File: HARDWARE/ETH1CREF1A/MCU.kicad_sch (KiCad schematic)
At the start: 42 parts, among them J1001 Conn_02x01, J1002 20021111-00010T4LF, U1001 HDC1080, U1002 STM32F746ZG, U1003 24LC08B-E/MS, Y1001 NX5032GA-16.000M

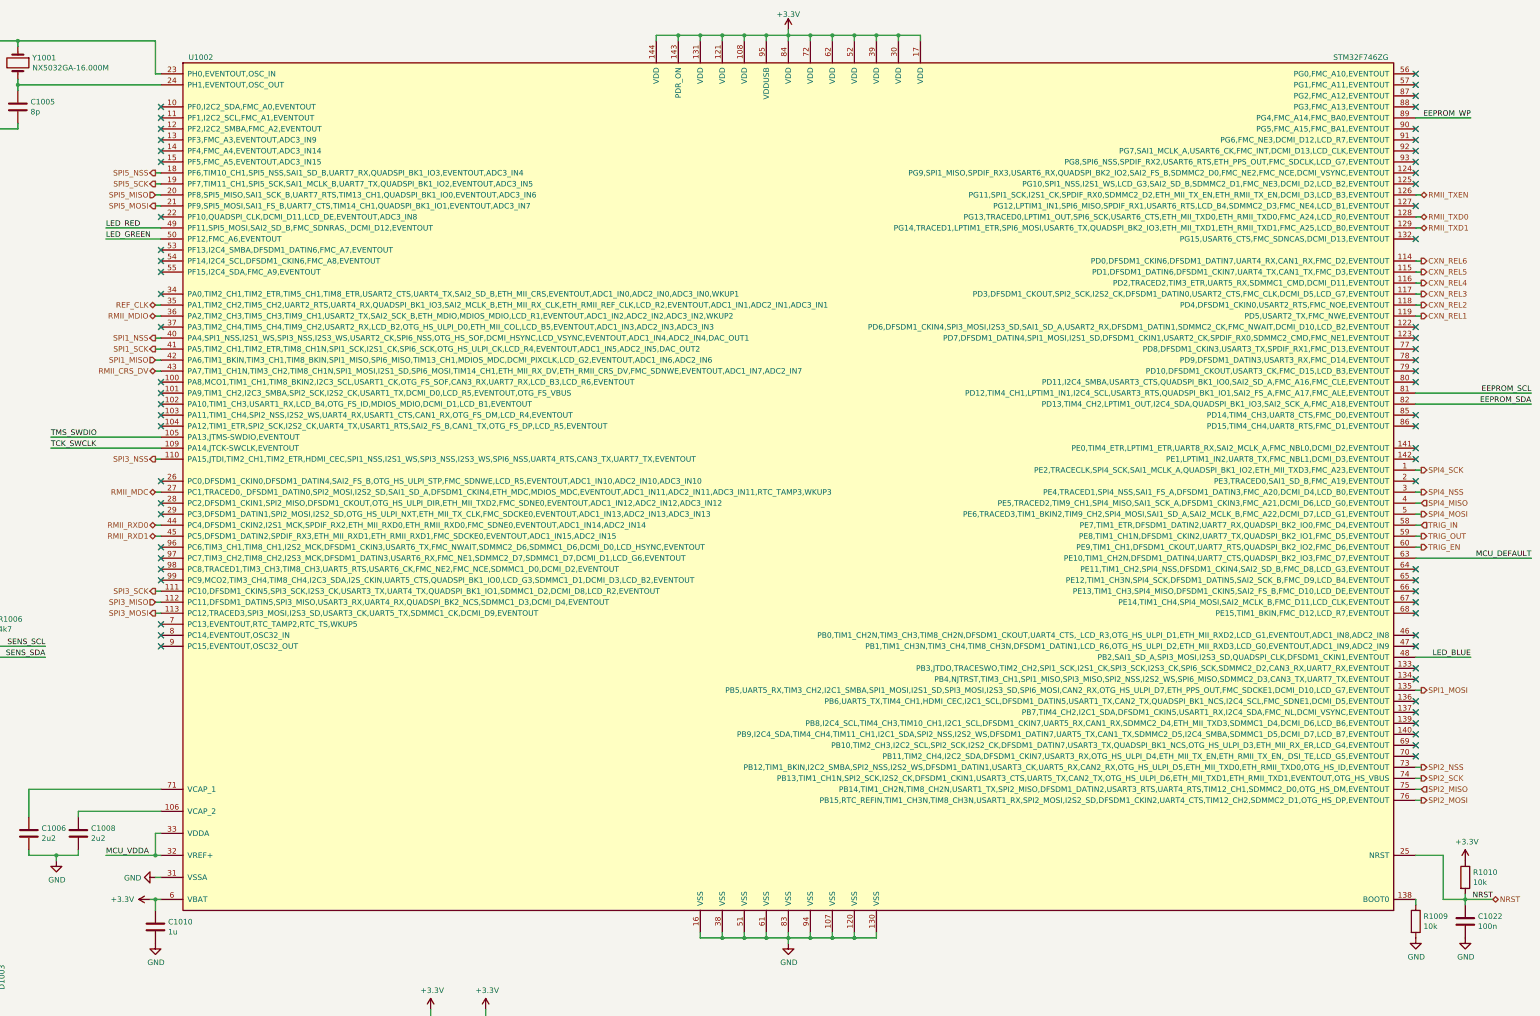
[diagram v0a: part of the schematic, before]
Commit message: Hardware and software
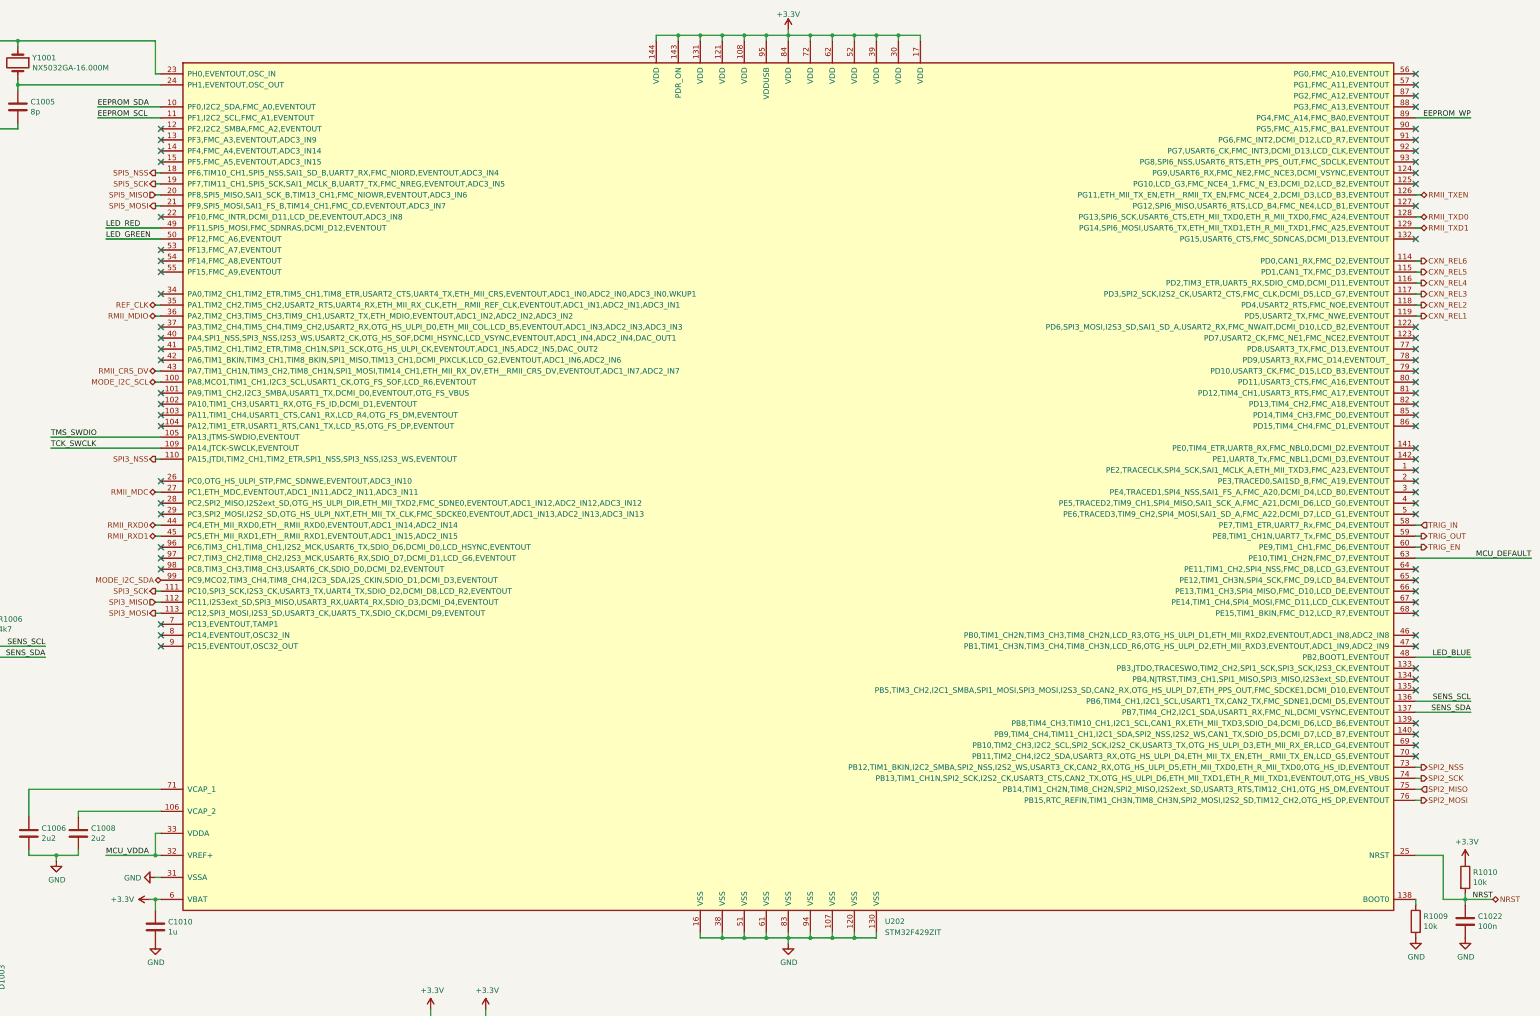
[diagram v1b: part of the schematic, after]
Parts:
- removed U1002: STM32F746ZG, ETH1CREF1A:TQFP-144_20x20mm_P0.5mm, symbol ETH1CSMU2:STM32F746ZG
- added U202: STM32F429ZIT, ETH1CREF1A:TQFP-144_20x20mm_P0.5mm, symbol ETH1CREF1A:STM32F429ZIT
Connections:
- net +3.3V: now also U202.108 (VDD), U202.121 (VDD), U202.131 (VDD), U202.143 (PDR_ON), U202.144 (VDD), U202.17 (VDD), U202.30 (VDD), U202.39 (VDD), U202.52 (VDD), U202.6 (VBAT), U202.62 (VDD), U202.72 (VDD), U202.84 (VDD), U202.95 (VDDUSB)
- net CXN_REL1: now also U202.119 (PD5,USART2_TX,FMC_NWE,EVENTOUT)
- net CXN_REL2: now also U202.118 (PD4,USART2_RTS,FMC_NOE,EVENTOUT)
- net CXN_REL3: now also U202.117 (PD3,SPI2_SCK,I2S2_CK,USART2_CTS,FMC_CLK,DCMI_D5,LCD_G7,EVENTOUT)
- net CXN_REL4: now also U202.116 (PD2,TIM3_ETR,UART5_RX,SDIO_CMD,DCMI_D11,EVENTOUT)
- net CXN_REL5: now also U202.115 (PD1,CAN1_TX,FMC_D3,EVENTOUT)
- net CXN_REL6: now also U202.114 (PD0,CAN1_RX,FMC_D2,EVENTOUT)
- net EEPROM_SCL: now also U202.11 (PF1,I2C2_SCL,FMC_A1,EVENTOUT)
- net EEPROM_SDA: now also U202.10 (PF0,I2C2_SDA,FMC_A0,EVENTOUT)
- net EEPROM_WP: now also U202.89 (PG4,FMC_A14,FMC_BA0,EVENTOUT)
- net GND: now also U202.107 (VSS), U202.120 (VSS), U202.130 (VSS), U202.16 (VSS), U202.31 (VSSA), U202.38 (VSS), U202.51 (VSS), U202.61 (VSS), U202.83 (VSS), U202.94 (VSS)
- net LED_BLUE: now also U202.48 (PB2,BOOT1,EVENTOUT)
- net LED_GREEN: now also U202.50 (PF12,FMC_A6,EVENTOUT)
- net LED_RED: now also U202.49 (PF11,SPI5_MOSI,FMC_SDNRAS,DCMI_D12,EVENTOUT)
- net MCU_DEFAULT: now also U202.63 (PE10,TIM1_CH2N,FMC_D7,EVENTOUT)
- net MCU_VDDA: now also U202.32 (VREF+), U202.33 (VDDA)
- net NRST: now also U202.25 (NRST)
- net REF_CLK: now also U202.35 (PA1,TIM2_CH2,TIM5_CH2,USART2_RTS,UART4_RX,ETH_MII_RX_CLK,ETH__RMII_REF_CLK,EVENTOUT,ADC1_IN1,ADC2_IN1,ADC3_IN1)
- net RMII_CRS_DV: now also U202.43 (PA7,TIM1_CH1N,TIM3_CH2,TIM8_CH1N,SPI1_MOSI,TIM14_CH1,ETH_MII_RX_DV,ETH__RMII_CRS_DV,EVENTOUT,ADC1_IN7,ADC2_IN7)
- net RMII_MDC: now also U202.27 (PC1,ETH_MDC,EVENTOUT,ADC1_IN11,ADC2_IN11,ADC3_IN11)
- net RMII_MDIO: now also U202.36 (PA2,TIM2_CH3,TIM5_CH3,TIM9_CH1,USART2_TX,ETH_MDIO,EVENTOUT,ADC1_IN2,ADC2_IN2,ADC3_IN2)
- net RMII_RXD0: now also U202.44 (PC4,ETH_MII_RXD0,ETH__RMII_RXD0,EVENTOUT,ADC1_IN14,ADC2_IN14)
- net RMII_RXD1: now also U202.45 (PC5,ETH_MII_RXD1,ETH__RMII_RXD1,EVENTOUT,ADC1_IN15,ADC2_IN15)
- net RMII_TXD0: now also U202.128 (PG13,SPI6_SCK,USART6_CTS,ETH_MII_TXD0,ETH_R_MII_TXD0,FMC_A24,EVENTOUT)
- net RMII_TXD1: now also U202.129 (PG14,SPI6_MOSI,USART6_TX,ETH_MII_TXD1,ETH_R_MII_TXD1,FMC_A25,EVENTOUT)
- net RMII_TXEN: now also U202.126 (PG11,ETH_MII_TX_EN,ETH__RMII_TX_EN,FMC_NCE4_2,DCMI_D3,LCD_B3,EVENTOUT)
- net SENS_SCL: now also U202.136 (PB6,TIM4_CH1,I2C1_SCL,USART1_TX,CAN2_TX,FMC_SDNE1,DCMI_D5,EVENTOUT)
- net SENS_SDA: now also U202.137 (PB7,TIM4_CH2,I2C1_SDA,USART1_RX,FMC_NL,DCMI_VSYNC,EVENTOUT)
- net SPI2_MISO: now also U202.75 (PB14,TIM1_CH2N,TIM8_CH2N,SPI2_MISO,I2S2ext_SD,USART3_RTS,TIM12_CH1,OTG_HS_DM,EVENTOUT)
- net SPI2_MOSI: now also U202.76 (PB15,RTC_REFIN,TIM1_CH3N,TIM8_CH3N,SPI2_MOSI,I2S2_SD,TIM12_CH2,OTG_HS_DP,EVENTOUT)
- net SPI2_NSS: now also U202.73 (PB12,TIM1_BKIN,I2C2_SMBA,SPI2_NSS,I2S2_WS,USART3_CK,CAN2_RX,OTG_HS_ULPI_D5,ETH_MII_TXD0,ETH_R_MII_TXD0,OTG_HS_ID,EVENTOUT)
- net SPI2_SCK: now also U202.74 (PB13,TIM1_CH1N,SPI2_SCK,I2S2_CK,USART3_CTS,CAN2_TX,OTG_HS_ULPI_D6,ETH_MII_TXD1,ETH_R_MII_TXD1,EVENTOUT,OTG_HS_VBUS)
- net SPI3_MISO: now also U202.112 (PC11,I2S3ext_SD,SPI3_MISO,USART3_RX,UART4_RX,SDIO_D3,DCMI_D4,EVENTOUT)
- net SPI3_MOSI: now also U202.113 (PC12,SPI3_MOSI,I2S3_SD,USART3_CK,UART5_TX,SDIO_CK,DCMI_D9,EVENTOUT)
- net SPI3_NSS: now also U202.110 (PA15,JTDI,TIM2_CH1,TIM2_ETR,SPI1_NSS,SPI3_NSS,I2S3_WS,EVENTOUT)
- net SPI3_SCK: now also U202.111 (PC10,SPI3_SCK,I2S3_CK,USART3_TX,UART4_TX,SDIO_D2,DCMI_D8,LCD_R2,EVENTOUT)
- net SPI5_MISO: now also U202.20 (PF8,SPI5_MISO,SAI1_SCK_B,TIM13_CH1,FMC_NIOWR,EVENTOUT,ADC3_IN6)
- net SPI5_MOSI: now also U202.21 (PF9,SPI5_MOSI,SAI1_FS_B,TIM14_CH1,FMC_CD,EVENTOUT,ADC3_IN7)
- net SPI5_NSS: now also U202.18 (PF6,TIM10_CH1,SPI5_NSS,SAI1_SD_B,UART7_RX,FMC_NIORD,EVENTOUT,ADC3_IN4)
- net SPI5_SCK: now also U202.19 (PF7,TIM11_CH1,SPI5_SCK,SAI1_MCLK_B,UART7_TX,FMC_NREG,EVENTOUT,ADC3_IN5)
- net TCK_SWCLK: now also U202.109 (PA14,JTCK-SWCLK,EVENTOUT)
- net TMS_SWDIO: now also U202.105 (PA13,JTMS-SWDIO,EVENTOUT)
- net TRIG_EN: now also U202.60 (PE9,TIM1_CH1,FMC_D6,EVENTOUT)
- net TRIG_IN: now also U202.58 (PE7,TIM1_ETR,UART7_Rx,FMC_D4,EVENTOUT)
- net TRIG_OUT: now also U202.59 (PE8,TIM1_CH1N,UART7_Tx,FMC_D5,EVENTOUT)
- net at C1003.1, Y1001.1: now also U202.23 (PH0,EVENTOUT,OSC_IN)
- net at C1005.1, Y1001.2: now also U202.24 (PH1,EVENTOUT,OSC_OUT)
- net at R1009.1: now also U202.138 (BOOT0)
- net at C1006.1: now also U202.71 (VCAP_1)
- net at C1008.1: now also U202.106 (VCAP_2)
- new net MODE_I2C_SCL: U202.100 (PA8,MCO1,TIM1_CH1,I2C3_SCL,USART1_CK,OTG_FS_SOF,LCD_R6,EVENTOUT)
- new net MODE_I2C_SDA: U202.99 (PC9,MCO2,TIM3_CH4,TIM8_CH4,I2C3_SDA,I2S_CKIN,SDIO_D1,DCMI_D3,EVENTOUT)
- no-connect marks 69 -> 73
